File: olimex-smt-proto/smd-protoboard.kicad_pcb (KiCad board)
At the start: 2 copper layers, 124.5 x 101.6 mm, 101 parts

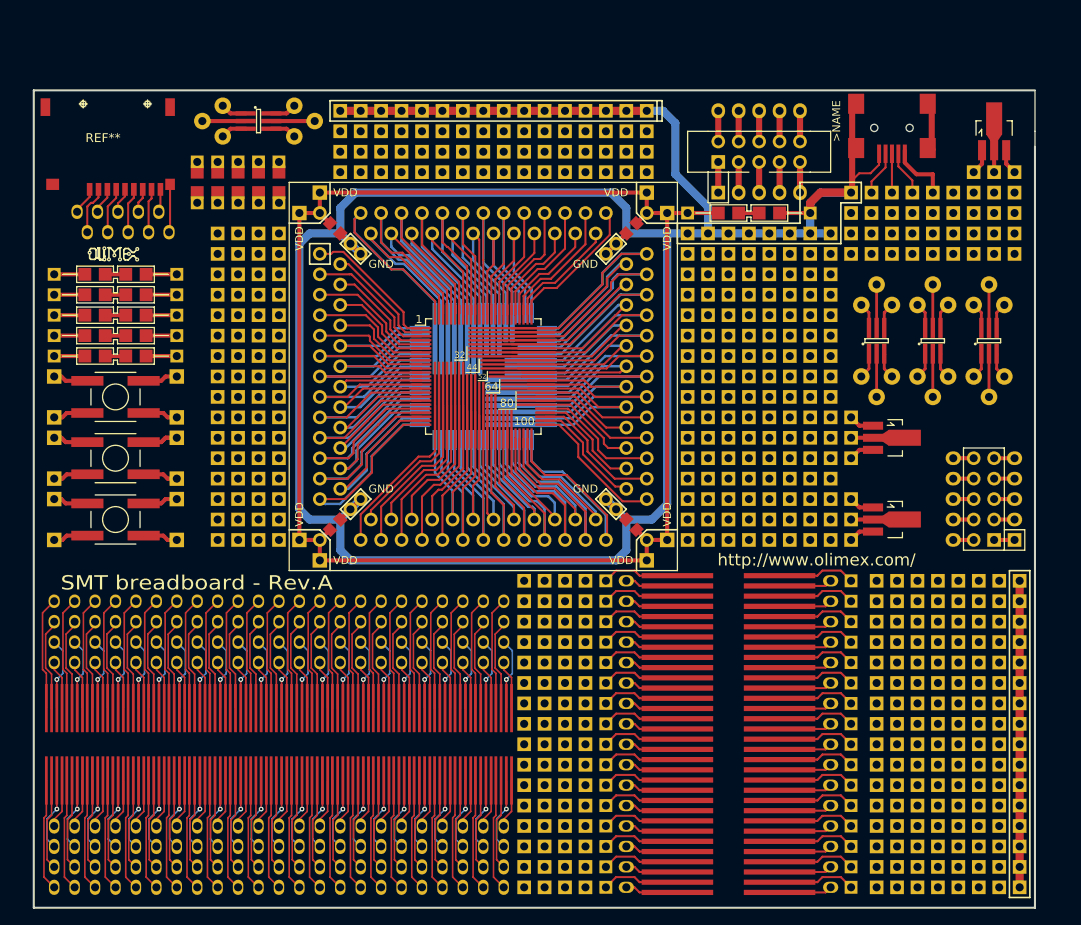
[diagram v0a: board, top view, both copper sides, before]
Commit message: initial commit
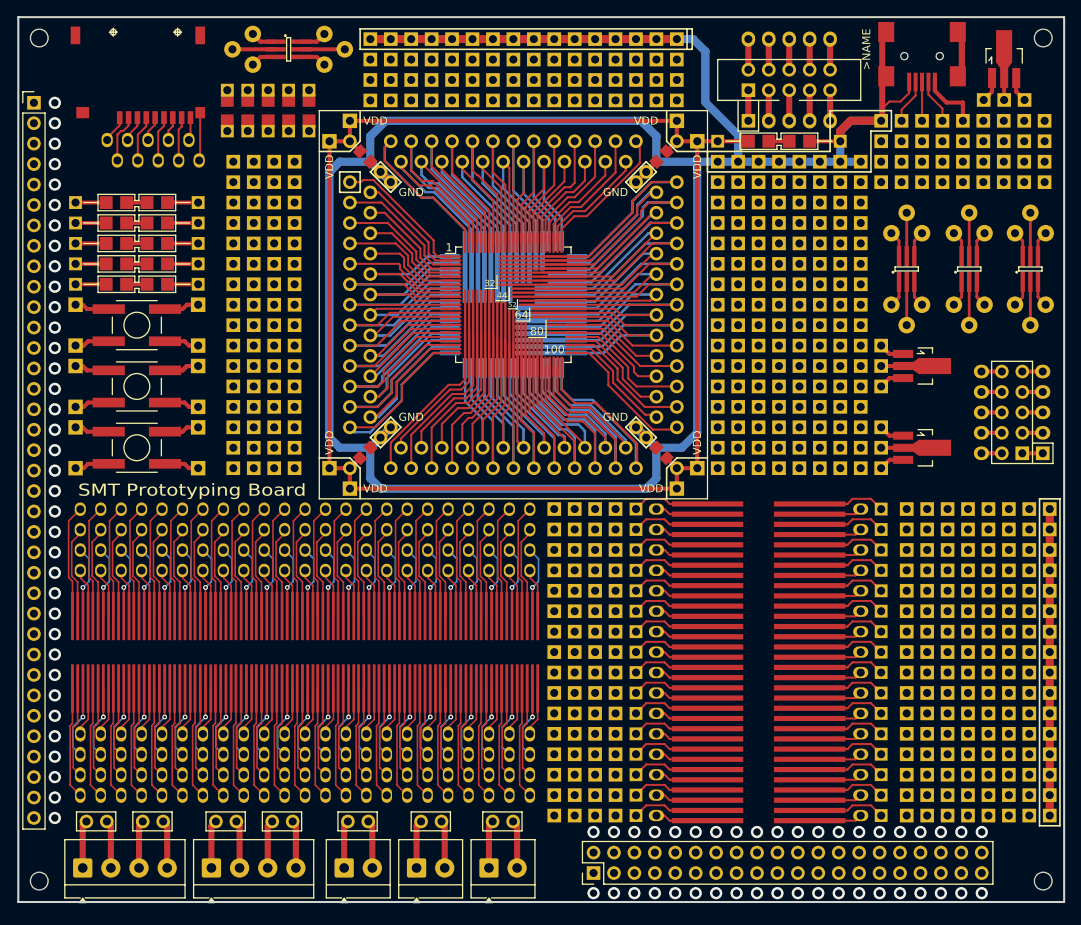
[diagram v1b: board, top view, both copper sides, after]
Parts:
- removed the >NAME at (188.0, 52.1)
- removed the ? at (137.2, 83.8)
- removed the ? at (162.6, 104.1)
- removed the ? at (104.1, 73.7)
- removed the ? at (104.1, 83.8)
- removed the ? at (104.1, 94.0)
- removed the ? at (104.1, 104.1)
- removed the ? at (186.1, 147.3)
- removed the ? at (186.1, 137.2)
- removed the ? at (186.1, 127.0)
- removed the ? at (186.1, 116.8)
- removed the ? at (91.4, 81.3)
- removed the ? at (91.4, 101.6)
- removed the ? at (101.6, 59.7)
- removed the ? at (104.1, 59.7)
- removed the ? at (106.7, 59.7)
- removed the ? at (109.2, 59.7)
- removed the ? at (111.8, 59.7)
- removed the ? at (167.6, 109.2)
- removed the ? at (167.6, 111.8)
- removed the ? at (167.6, 116.8)
- removed the ? at (167.6, 114.3)
- removed the ? at (167.6, 124.5)
- removed the ? at (119.4, 58.4)
- removed the ? at (167.6, 127.0)
- removed the ? at (167.6, 121.9)
- removed the ? at (167.6, 119.4)
- removed the ? at (167.6, 139.7)
- removed the ? at (167.6, 142.2)
- removed the ? at (167.6, 147.3)
- removed the ? at (167.6, 144.8)
- removed the ? at (167.6, 134.6)
- removed the ? at (167.6, 137.2)
- removed the ? at (167.6, 132.1)
- removed the ? at (129.5, 58.4)
- removed the ? at (167.6, 129.5)
- removed the ? at (86.4, 129.5)
- removed the ? at (83.8, 129.5)
- removed the ? at (88.9, 129.5)
- removed the ? at (91.4, 129.5)
- removed the ? at (101.6, 129.5)
- removed the ? at (99.1, 129.5)
- removed the ? at (94.0, 129.5)
- removed the ? at (96.5, 129.5)
- removed the ? at (116.8, 129.5)
- removed the ? at (139.7, 58.4)
- removed the ? at (114.3, 129.5)
- removed the ? at (119.4, 129.5)
- removed the ? at (121.9, 129.5)
- removed the ? at (111.8, 129.5)
- removed the ? at (109.2, 129.5)
- removed the ? at (104.1, 129.5)
- removed the ? at (106.7, 129.5)
- removed the ? at (137.2, 129.5)
- removed the ? at (134.6, 129.5)
- removed the ? at (139.7, 129.5)
- removed the ? at (149.9, 58.4)
- removed the ? at (132.1, 129.5)
- removed the ? at (129.5, 129.5)
- removed the ? at (124.5, 129.5)
- removed the ? at (127.0, 129.5)
- removed the ? at (91.4, 94.0)
- removed the ? at (91.4, 86.4)
- removed the ? at (91.4, 78.7)
- removed the ? at (91.4, 73.7)
- removed the ? at (91.4, 76.2)
- removed the ? at (200.0, 79.4)
- removed the ? at (162.6, 73.7)
- removed the ? at (186.1, 79.4)
- removed the ? at (170.2, 63.5)
- removed the ? at (200.7, 53.3)
- removed the ? at (188.0, 101.6)
- removed the ? at (188.0, 91.4)
- removed the ? at (193.0, 79.4)
- removed the ? at (172.7, 73.7)
- removed the ? at (172.7, 83.8)
- removed the ? at (172.7, 94.0)
- removed the ? at (172.7, 104.1)
- removed the ? at (162.6, 83.8)
- removed the ? at (200.7, 104.1)
- removed the ? at (166.4, 57.1)
- removed the ? at (109.2, 52.1)
- removed the ? at (90.5, 53.2)
- removed the ? at (91.4, 71.1)
- removed the ? at (195.6, 68.6)
- removed the ? at (182.9, 61.0)
- removed the ? at (142.2, 116.8)
- removed the ? at (142.2, 127.0)
- removed the ? at (142.2, 137.2)
- removed the ? at (162.6, 94.0)
- removed the ? at (142.2, 147.3)
- removed the ? at (196.2, 147.3)
- removed the ? at (196.2, 137.2)
- removed the ? at (196.2, 127.0)
- removed the ? at (196.2, 116.8)
- removed the G*** at (167.7, 127.7)
- removed the OLIMEX_LOGO** at (167.4, 114.8)
- removed the REF** at (91.2, 68.6)
- removed the REF** at (137.2, 83.8)
- removed the REF** at (95.0, 131.3)
- removed RoHS: Compliant, OLIMEX_LOGOs-FP:LOGO_ROHS_1
- added >NAME: >VALUE, Proto:USB_Mini-B-NOSILK, F.Cu at (191.7, 43.1)
- added ?: , Proto:Proto_Grid_4x4_2.54mm_Square, F.Cu at (106.1, 64.7)
- added ?: , Proto:Proto_SSOP_0.65, F.Cu at (92.1, 118.1)
- added ?: , Proto:Proto_Tactile_Button, F.Cu at (94.1, 85.1)
- added ?: , Proto:Proto_SOT-23-6, F.Cu at (189.8, 70.5)
- added ?: , Proto:Proto_1206_Pads_x2_LED_HandSolder, F.Cu at (94.1, 69.8)
- added ?: , Proto:Proto_SSOP_0.65, F.Cu at (115.0, 118.1)
- added ?: , Proto:Proto_conn_2x5_JTAG, F.Cu at (204.2, 93.4)
- added ?: , Proto:Proto_Grid_4x4_2.54mm_Square, F.Cu at (146.0, 138.4)
- added ?: , Proto:Proto_SSOP_0.65, F.Cu at (107.4, 118.1)
- added ?: , Proto:Proto_Grid_4x4_2.54mm_Square, F.Cu at (123.1, 49.5)
- added ?: , Proto:Proto_Grid_4x4_2.54mm_Square, F.Cu at (176.5, 95.2)
- added ?: , Proto:Proto_SOT-23-6, F.Cu at (197.6, 70.5)
- added ?: , Proto:Proto_Tactile_Button, F.Cu at (94.1, 92.7)
- added ?: , Proto:Proto_Grid_4x4_2.54mm_Square, F.Cu at (166.3, 74.9)
- added ?: , Proto:Proto_SOIC_1.27mm, F.Cu at (171.4, 135.9)
- added ?: , Proto:Proto_SSOP_0.65, F.Cu at (120.1, 118.1)
- added ?: , Proto:Proto_Grid_4x4_2.54mm_Square, F.Cu at (106.1, 95.2)
- added ?: , Proto:Proto_SOIC_1.27mm, F.Cu at (171.4, 138.4)
- added ?: , Proto:Proto_Conn_TFC-WPAPR-08, F.Cu at (94.2, 44.3)
- added ?: , Proto:Proto_1206_Pads_x2_LED_HandSolder, F.Cu at (173.9, 54.6)
- added ?: , Proto:Proto_1206_Pads_x2_LED_HandSolder, F.Cu at (94.1, 64.7)
- added ?: , Proto:Proto_Grid_4x4_2.54mm_Square, F.Cu at (133.3, 49.5)
- added ?: , Proto:Proto_0805_Pads_Compact, F.Cu at (105.3, 50.8)
- added ?: , Proto:Proto_Grid_4x4_2.54mm_Square, F.Cu at (166.3, 95.2)
- added ?: , Proto:Proto_conn_2x5_UEXT-M, F.Cu at (170.1, 48.2)
- added ?: , Proto:Proto_SOIC_1.27mm, F.Cu at (171.4, 100.3)
- added ?: , Proto:Proto_Grid_4x4_2.54mm_Square, F.Cu at (200.0, 128.2)
- added ?: , Proto:Proto_Grid_4x4_2.54mm_Square, F.Cu at (199.3, 59.7)
- added ?: , Proto:Proto_Grid_4x4_2.54mm_Square, F.Cu at (176.5, 74.9)
- added ?: , Proto:Proto_SOIC_1.27mm, F.Cu at (171.4, 110.5)
- added ?: , Proto:Proto_SSOP_0.65, F.Cu at (122.6, 118.1)
- added ?: , Proto:Proto_SOIC_1.27mm, F.Cu at (171.4, 133.3)
- added ?: , Proto:Proto_Grid_4x4_2.54mm_Square, F.Cu at (146.0, 118.1)
- added ?: , Proto:Proto_SOT89-3, F.Cu at (191.7, 92.7)
- added ?: , Proto:Proto_SOIC_1.27mm, F.Cu at (171.4, 105.4)
- added ?: , Proto:Proto_Grid_4x4_2.54mm_Square, F.Cu at (189.8, 118.1)
- added ?: , Proto:Proto_Grid_4x4_2.54mm_Square, F.Cu at (200.0, 118.1)
- added ?: , Proto:Proto_1206_Pads_x2_LED_HandSolder, F.Cu at (94.1, 67.3)
- added ?: , Proto:Proto_SSOP_0.65, F.Cu at (132.8, 118.1)
- added ?: , Proto:Proto_Grid_4x4_2.54mm_Square, F.Cu at (176.5, 85.1)
- added ?: , Proto:Proto_SSOP_0.65, F.Cu at (127.7, 118.1)
- added ?: , Proto:Proto_SOIC_1.27mm, F.Cu at (171.4, 125.7)
- added ?: , Proto:Proto_Grid_4x4_2.54mm_Square, F.Cu at (106.1, 74.9)
- added ?: , Proto:Proto_SSOP_0.65, F.Cu at (117.5, 118.1)
- added ?: , Proto:Proto_Grid_4x4_2.54mm_Square, F.Cu at (200.0, 138.4)
- added ?: , Proto:Proto_1206_Pads_x2_LED_HandSolder, F.Cu at (94.1, 72.4)
- added ?: , Proto:Proto_SOIC_1.27mm, F.Cu at (171.4, 123.2)
- added ?: , Proto:Proto_SSOP_0.65, F.Cu at (99.8, 118.1)
- added ?: , Proto:Proto_SOIC_1.27mm, F.Cu at (171.4, 113.0)
- added ?: , Proto:Proto_SOT-23-6, F.Cu at (205.2, 70.5)
- added ?: , Proto:Proto_TQFP_upto100_0.50, F.Cu at (140.9, 74.9)
- added ?: , Proto:Proto_Grid_4x4_2.54mm_Square, F.Cu at (146.0, 107.9)
- added ?: , Proto:Proto_Grid_4x4_2.54mm_Square, F.Cu at (189.8, 138.4)
- added ?: , Proto:Proto_Grid_4x4_2.54mm_Square, F.Cu at (153.6, 49.5)
- added ?: , Proto:Proto_0805_Pads_Compact, F.Cu at (107.9, 50.8)
- added ?: , Proto:Proto_Grid_4x4_2.54mm_Square, F.Cu at (166.3, 85.1)
- added ?: , Proto:Proto_SSOP_0.65, F.Cu at (97.2, 118.1)
- added ?: , Proto:Proto_SOT-23-6, F.Cu at (113.0, 43.1)
- added ?: , Proto:Proto_SOT89-3, F.Cu at (201.9, 44.4)
- added ?: , Proto:Proto_SSOP_0.65, F.Cu at (137.9, 118.1)
- added ?: , Proto:Proto_SSOP_0.65, F.Cu at (104.8, 118.1)
- added ?: , Proto:Proto_Grid_4x4_2.54mm_Square, F.Cu at (106.1, 85.1)
- added ?: , Proto:Proto_Tactile_Button, F.Cu at (94.1, 77.4)
- added ?: , Proto:Proto_0805_Pads_Compact, F.Cu at (110.4, 50.8)
- added ?: , Proto:Proto_SSOP_0.65, F.Cu at (142.9, 118.1)
- added ?: , Proto:Proto_Grid_4x4_2.54mm_Square, F.Cu at (189.8, 107.9)
- added ?: , Proto:Proto_Grid_4x4_2.54mm_Square, F.Cu at (200.0, 107.9)
- added ?: , Proto:Proto_SSOP_0.65, F.Cu at (94.7, 118.1)
- added ?: , Proto:Proto_SOIC_1.27mm, F.Cu at (171.4, 130.8)
- added ?: , Proto:Proto_SOT89-3, F.Cu at (191.7, 82.5)
- added ?: , Proto:Proto_SOIC_1.27mm, F.Cu at (171.4, 107.9)
- added ?: , Proto:Proto_SOIC_1.27mm, F.Cu at (171.4, 128.2)
- added ?: , Proto:Proto_SOIC_1.27mm, F.Cu at (171.4, 118.1)
- added ?: , Proto:Proto_SSOP_0.65, F.Cu at (109.9, 118.1)
- added ?: , Proto:Proto_Grid_5x4_2.54mm_Square, F.Cu at (186.6, 52.0)
- added ?: , Proto:Proto_SSOP_0.65, F.Cu at (89.6, 118.1)
- added ?: , Proto:Proto_SOIC_1.27mm, F.Cu at (171.4, 102.8)
- added ?: , Proto:Proto_Grid_4x4_2.54mm_Square, F.Cu at (143.4, 49.5)
- added ?: , Proto:Proto_SSOP_0.65, F.Cu at (102.3, 118.1)
- added ?: , Proto:Proto_0805_Pads_Compact, F.Cu at (115.5, 50.8)
- added ?: , Proto:Proto_Grid_4x4_2.54mm_Square, F.Cu at (189.8, 128.2)
- added ?: , Proto:Proto_SSOP_0.65, F.Cu at (135.3, 118.1)
- added ?: , Proto:Proto_SSOP_0.65, F.Cu at (87.1, 118.1)
- added ?: , Proto:Proto_SSOP_0.65, F.Cu at (112.5, 118.1)
- added ?: , Proto:Proto_SSOP_0.65, F.Cu at (130.2, 118.1)
- added ?: , Proto:Proto_SOIC_1.27mm, F.Cu at (171.4, 115.5)
- added ?: , Proto:Proto_1206_Pads_x2_LED_HandSolder, F.Cu at (94.1, 62.2)
- added ?: , Proto:Proto_Grid_4x4_2.54mm_Square, F.Cu at (166.3, 64.7)
- added ?: , Proto:Proto_SSOP_0.65, F.Cu at (140.4, 118.1)
- added ?: , Proto:Proto_SOIC_1.27mm, F.Cu at (171.4, 120.6)
- added ?: , Proto:Proto_0805_Pads_Compact, F.Cu at (113.0, 50.8)
- added ?: , Proto:Proto_Grid_4x4_2.54mm_Square, F.Cu at (176.5, 64.7)
- added ?: , Proto:Proto_Grid_4x4_2.54mm_Square, F.Cu at (146.0, 128.2)
- added ?: , Proto:Proto_SSOP_0.65, F.Cu at (125.2, 118.1)
- added G***: LOGO, Proto:LOGO_OSHW_600, B.Cu at (171.5, 122.5)
- added G***: LOGO, kml-custom:FAST-Logo-Large, B.Cu at (171.4, 105.2)
- added OLIMEX_LOGO**: OLIMEX_LOGO_TB, Proto:OLIMEX_LOGO_TB, B.Cu at (171.3, 136.8)
- added REF**: TerminalBlock_4Ucon_1x02_P3.50mm_Horizontal, TerminalBlock_4Ucon:TerminalBlock_4Ucon_1x02_P3.50mm_Horizontal, F.Cu at (137.9, 144.9)
- added REF**: Proto_Pins_2_P2.54mm, Proto:Proto_Pins_2_P2.54mm, F.Cu at (139.6, 139.1)
- added REF**: TerminalBlock_4Ucon_1x04_P3.50mm_Horizontal, TerminalBlock_4Ucon:TerminalBlock_4Ucon_1x04_P3.50mm_Horizontal, F.Cu at (87.4, 144.9)
- added REF**: Proto_Pins_2_P2.54mm, Proto:Proto_Pins_2_P2.54mm, F.Cu at (130.7, 139.1)
- added REF**: Proto_Pins_2_P2.54mm, Proto:Proto_Pins_2_P2.54mm, F.Cu at (121.6, 139.1)
- added REF**: TerminalBlock_4Ucon_1x02_P3.50mm_Horizontal, TerminalBlock_4Ucon:TerminalBlock_4Ucon_1x02_P3.50mm_Horizontal, F.Cu at (128.9, 144.9)
- added REF**: MountingHole_2.2mm_M2, MountingHole:MountingHole_2.2mm_M2, F.Cu at (206.8, 41.7)
- added REF**: MountingHole_2.2mm_M2, MountingHole:MountingHole_2.2mm_M2, F.Cu at (82.0, 41.7)
- added REF**: Proto_Pins_2_P2.54mm, Proto:Proto_Pins_2_P2.54mm, F.Cu at (89.1, 139.1)
- added REF**: MountingHole_2.2mm_M2, MountingHole:MountingHole_2.2mm_M2, F.Cu at (82.0, 146.5)
- added REF**: LQFP-64_14x14mm_0.8mm, Proto:Proto_LQFP_upto64_0.8mm, B.Cu at (140.9, 74.9)
- added REF**: PinHeader_2x20_P2.54mm_Vertical, Connector_PinHeader_2.54mm:PinHeader_2x20_P2.54mm_Vertical, F.Cu at (150.9, 145.5)
- added REF**: TerminalBlock_4Ucon_1x04_P3.50mm_Horizontal, TerminalBlock_4Ucon:TerminalBlock_4Ucon_1x04_P3.50mm_Horizontal, F.Cu at (103.4, 144.9)
- added REF**: Proto_Pins_2_P2.54mm, Proto:Proto_Pins_2_P2.54mm, F.Cu at (112.2, 139.1)
- added REF**: PinHeader_1x36_P2.54mm_Vertical, Connector_PinHeader_2.54mm:PinHeader_1x36_P2.54mm_Vertical, F.Cu at (81.3, 49.8)
- added REF**: TerminalBlock_4Ucon_1x02_P3.50mm_Horizontal, TerminalBlock_4Ucon:TerminalBlock_4Ucon_1x02_P3.50mm_Horizontal, F.Cu at (119.9, 144.9)
- added REF**: Proto_Pins_2_P2.54mm, Proto:Proto_Pins_2_P2.54mm, F.Cu at (105.2, 139.1)
- added REF**: Proto_Pins_2_P2.54mm, Proto:Proto_Pins_2_P2.54mm, F.Cu at (96.1, 139.1)
- added REF**: MountingHole_2.2mm_M2, MountingHole:MountingHole_2.2mm_M2, F.Cu at (206.8, 146.5)
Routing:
- net (no net): track 5752.1 -> 5835.7 mm, vias 46 -> 122
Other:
- board size 124.5 x 101.6 mm -> 130 x 110 mm
- board text added: "Originally by..."
- board text added: "SMT Prototyping Board"
- board text removed: "SMT breadboard - Rev.A"
- board text removed: "http://www.olimex.com/"
